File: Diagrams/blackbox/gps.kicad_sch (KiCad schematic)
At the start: 1 part, among them U7 UBlox M6

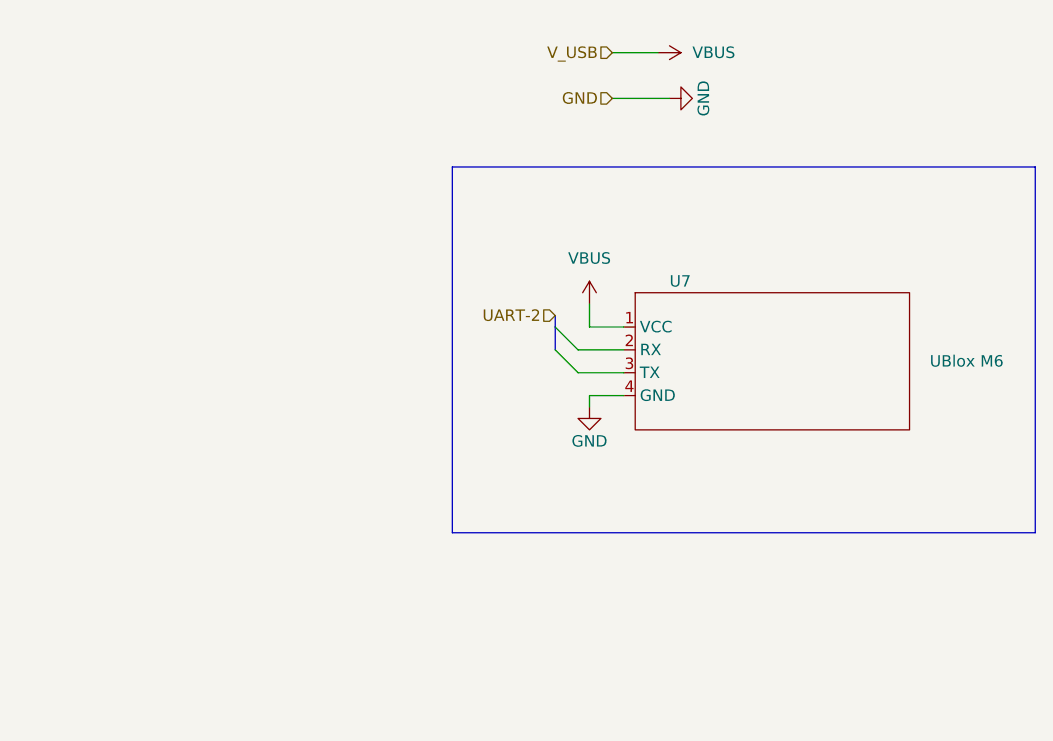
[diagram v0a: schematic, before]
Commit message: Blackbox Diagram V1.1
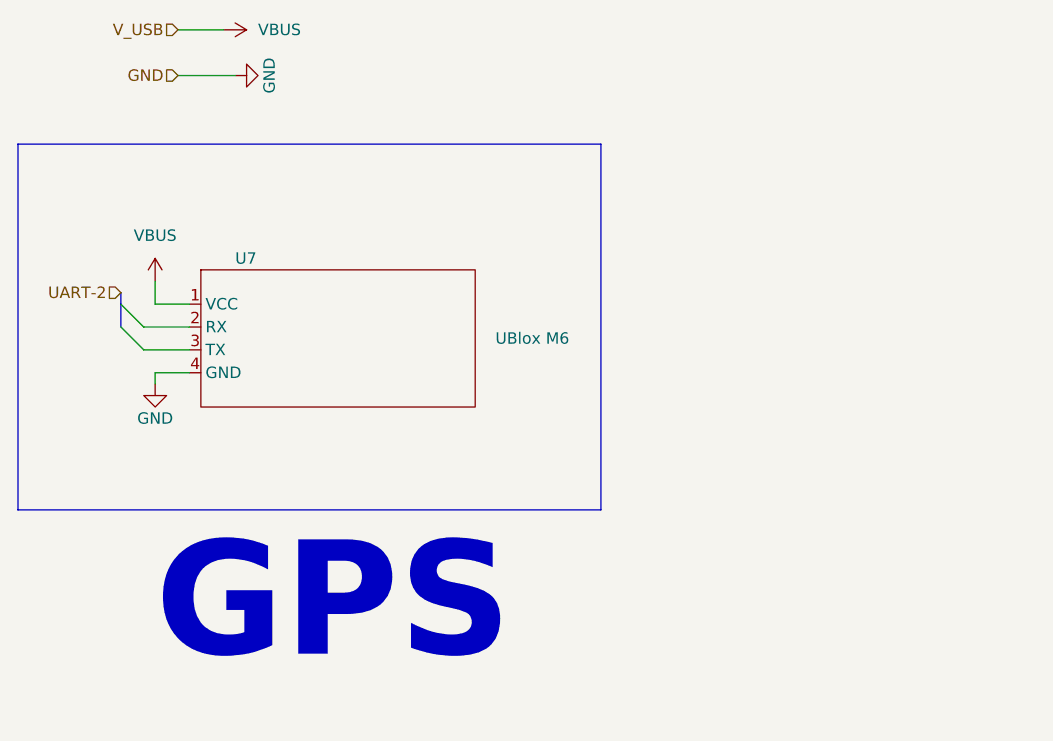
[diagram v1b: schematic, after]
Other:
- note added: "GPS"
- moved on the sheet: U7
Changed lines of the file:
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@@
     (comment 9 "TOLGA")
   )
-  (bus_entry (at 114.3 90.17) (size 2.54 2.54)
+  (bus_entry (at 66.04 87.63) (size 2.54 2.54)
     (stroke (width 0) (type default) (color 0 194 0 1))
   )
-  (bus_entry (at 114.3 87.63) (size 2.54 2.54)
+  (bus_entry (at 66.04 85.09) (size 2.54 2.54)
     (stroke (width 0) (type default) (color 0 0 194 1))
   )
-  (wire (pts (xy 118.11 85.09) (xy 118.11 87.63))
+  (wire (pts (xy 69.85 82.55) (xy 69.85 85.09))
     (stroke (width 0.5) (type default) (color 132 0 0 1))
   )
-  (wire (pts (xy 118.11 87.63) (xy 121.92 87.63))
+  (wire (pts (xy 69.85 85.09) (xy 73.66 85.09))
     (stroke (width 0.5) (type default) (color 132 0 0 1))
   )
-  (wire (pts (xy 116.84 92.71) (xy 121.92 92.71))
+  (wire (pts (xy 68.58 90.17) (xy 73.66 90.17))
     (stroke (width 0) (type default))
   )
-  (wire (pts (xy 120.65 62.23) (xy 127 62.23))
+  (wire (pts (xy 72.39 59.69) (xy 78.74 59.69))
     (stroke (width 0) (type default))
   )
-  (wire (pts (xy 118.11 95.25) (xy 118.11 96.52))
+  (wire (pts (xy 69.85 92.71) (xy 69.85 93.98))
     (stroke (width 0.5) (type default) (color 0 0 0 1))
   )
-  (wire (pts (xy 120.65 57.15) (xy 125.73 57.15))
+  (wire (pts (xy 72.39 54.61) (xy 77.47 54.61))
     (stroke (width 0) (type default))
   )
-  (bus (pts (xy 114.3 87.63) (xy 114.3 90.17))
+  (bus (pts (xy 66.04 85.09) (xy 66.04 87.63))
     (stroke (width 0) (type default))
   )
-  (bus (pts (xy 114.3 86.36) (xy 114.3 87.63))
+  (bus (pts (xy 66.04 83.82) (xy 66.04 85.09))
     (stroke (width 0) (type default))
   )
-  (wire (pts (xy 118.11 95.25) (xy 121.92 95.25))
+  (wire (pts (xy 69.85 92.71) (xy 73.66 92.71))
     (stroke (width 0.5) (type default) (color 0 0 0 1))
   )
-  (wire (pts (xy 116.84 90.17) (xy 121.92 90.17))
+  (wire (pts (xy 68.58 87.63) (xy 73.66 87.63))
     (stroke (width 0) (type default) (color 0 0 194 1))
   )
-  (rectangle (start 102.87 69.85) (end 167.64 110.49)
+  (rectangle (start 54.61 67.31) (end 119.38 107.95)
     (stroke (width 0) (type default))
     (fill (type none))
   )
-  (image (at 140.97 91.44) (scale 0.449707)
+  (image (at 92.71 88.9) (scale 0.449707)
     (data
       iVBORw0KGgoAAAANSUhEUgAAAZAAAAGQCAIAAAAP3aGbAAAAA3NCSVQICAjb4U/gAAAACXBIWXMA
@@
     )
   )
-  (hierarchical_label "GND" (shape input) (at 120.65 62.23 180) (fields_autoplaced)
+  (text "GPS" (at 69.85 125.73 0)
+    (effects (font (size 12.7 12.7) (thickness 2.54) bold) (justify left bottom))
+  )
+  (hierarchical_label "GND" (shape input) (at 72.39 59.69 180) (fields_autoplaced)
     (effects (font (size 1.27 1.27)) (justify right))
   )
-  (hierarchical_label "UART-2" (shape input) (at 114.3 86.36 180) (fields_autoplaced)
+  (hierarchical_label "UART-2" (shape input) (at 66.04 83.82 180) (fields_autoplaced)
     (effects (font (size 1.27 1.27)) (justify right))
   )
-  (hierarchical_label "V_USB" (shape input) (at 120.65 57.15 180) (fields_autoplaced)
+  (hierarchical_label "V_USB" (shape input) (at 72.39 54.61 180) (fields_autoplaced)
     (effects (font (size 1.27 1.27)) (justify right))
   )
-  (symbol (lib_id "power:GND") (at 118.11 96.52 0) (unit 1)
+  (symbol (lib_id "power:GND") (at 69.85 93.98 0) (unit 1)
     (in_bom yes) (on_board yes) (dnp no)
-    (property "Reference" "#PWR021" (at 118.11 102.87 0)
+    (property "Reference" "#PWR021" (at 69.85 100.33 0)
       (effects (font (size 1.27 1.27)) hide)
     )
-    (property "Value" "GND" (at 118.11 100.33 0)
+    (property "Value" "GND" (at 69.85 97.79 0)
       (effects (font (size 1.27 1.27)))
     )
-    (property "Footprint" "" (at 118.11 96.52 0)
+    (property "Footprint" "" (at 69.85 93.98 0)
       (effects (font (size 1.27 1.27)) hide)
     )
-    (property "Datasheet" "" (at 118.11 96.52 0)
+    (property "Datasheet" "" (at 69.85 93.98 0)
       (effects (font (size 1.27 1.27)) hide)
     )
@@
     )
   )
-  (symbol (lib_id "power:VBUS") (at 118.11 85.09 0) (unit 1)
+  (symbol (lib_id "power:VBUS") (at 69.85 82.55 0) (unit 1)
     (in_bom yes) (on_board yes) (dnp no) (fields_autoplaced)
-    (property "Reference" "#PWR019" (at 118.11 88.9 0)
+    (property "Reference" "#PWR019" (at 69.85 86.36 0)
       (effects (font (size 1.27 1.27)) hide)
     )
-    (property "Value" "VBUS" (at 118.11 80.01 0)
+    (property "Value" "VBUS" (at 69.85 77.47 0)
       (effects (font (size 1.27 1.27)))
     )
-    (property "Footprint" "" (at 118.11 85.09 0)
+    (property "Footprint" "" (at 69.85 82.55 0)
       (effects (font (size 1.27 1.27)) hide)
     )
-    (property "Datasheet" "" (at 118.11 85.09 0)
+    (property "Datasheet" "" (at 69.85 82.55 0)
       (effects (font (size 1.27 1.27)) hide)
     )
@@
     )
   )
-  (symbol (lib_id "power:VBUS") (at 125.73 57.15 270) (unit 1)
+  (symbol (lib_id "power:VBUS") (at 77.47 54.61 270) (unit 1)
     (in_bom yes) (on_board yes) (dnp no) (fields_autoplaced)
-    (property "Reference" "#PWR023" (at 121.92 57.15 0)
+    (property "Reference" "#PWR023" (at 73.66 54.61 0)
       (effects (font (size 1.27 1.27)) hide)
     )
-    (property "Value" "VBUS" (at 129.54 57.15 90)
+    (property "Value" "VBUS" (at 81.28 54.61 90)
       (effects (font (size 1.27 1.27)) (justify left))
     )
-    (property "Footprint" "" (at 125.73 57.15 0)
+    (property "Footprint" "" (at 77.47 54.61 0)
       (effects (font (size 1.27 1.27)) hide)
     )
-    (property "Datasheet" "" (at 125.73 57.15 0)
+    (property "Datasheet" "" (at 77.47 54.61 0)
       (effects (font (size 1.27 1.27)) hide)
     )
@@
     )
   )
-  (symbol (lib_name "Sparkfun_IMU_Razor_2") (lib_id "bitirme:Sparkfun_IMU_Razor") (at 123.19 83.82 0) (unit 1)
+  (symbol (lib_name "Sparkfun_IMU_Razor_2") (lib_id "bitirme:Sparkfun_IMU_Razor") (at 74.93 81.28 0) (unit 1)
     (in_bom yes) (on_board yes) (dnp no)
-    (property "Reference" "U7" (at 127 82.55 0)
+    (property "Reference" "U7" (at 78.74 80.01 0)
       (effects (font (size 1.27 1.27)) (justify left))
     )
-    (property "Value" "UBlox M6" (at 160.02 91.44 0)
+    (property "Value" "UBlox M6" (at 111.76 88.9 0)
       (effects (font (size 1.27 1.27)))
     )
-    (property "Footprint" "" (at 123.19 83.82 0)
+    (property "Footprint" "" (at 74.93 81.28 0)
       (effects (font (size 1.27 1.27)) hide)
     )
-    (property "Datasheet" "https://www.rlocman.ru/i/File/2011/04/22/1.pdf" (at 123.19 83.82 0)
+    (property "Datasheet" "https://www.rlocman.ru/i/File/2011/04/22/1.pdf" (at 74.93 81.28 0)
       (effects (font (size 1.27 1.27)) hide)
     )
-    (property "Website" "https://www.robotistan.com/gy-neo6mv2-gps-modulu-ucus-kontrol-sistem-gpsi" (at 123.19 83.82 0)
+    (property "Website" "https://www.robotistan.com/gy-neo6mv2-gps-modulu-ucus-kontrol-sistem-gpsi" (at 74.93 81.28 0)
       (effects (font (size 1.27 1.27)) hide)
     )
@@
     )
   )
-  (symbol (lib_id "power:GND") (at 127 62.23 90) (unit 1)
+  (symbol (lib_id "power:GND") (at 78.74 59.69 90) (unit 1)
     (in_bom yes) (on_board yes) (dnp no)
-    (property "Reference" "#PWR024" (at 133.35 62.23 0)
+    (property "Reference" "#PWR024" (at 85.09 59.69 0)
       (effects (font (size 1.27 1.27)) hide)
     )
-    (property "Value" "GND" (at 130.81 62.23 0)
+    (property "Value" "GND" (at 82.55 59.69 0)
       (effects (font (size 1.27 1.27)))
     )
-    (property "Footprint" "" (at 127 62.23 0)
+    (property "Footprint" "" (at 78.74 59.69 0)
       (effects (font (size 1.27 1.27)) hide)
     )
-    (property "Datasheet" "" (at 127 62.23 0)
+    (property "Datasheet" "" (at 78.74 59.69 0)
       (effects (font (size 1.27 1.27)) hide)
     )
